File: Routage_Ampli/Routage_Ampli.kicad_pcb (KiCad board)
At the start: 2 copper layers, 110.5 x 100.3 mm, 52 parts, among them J1 Conn_01x03, J2 Conn_01x02, Q1 2N2907, Q10 TIP32, Q11 BD138, Q12 TIP31, Q13 2N2222, Q2 2N2907, Q3 2N2907, Q4 2N2222, Q5 2N2222, Q6 2N2907, Q7 2N2907, Q8 BD139, Q9 BD139, U1 Jack_Mono, U2 Relay_1CT

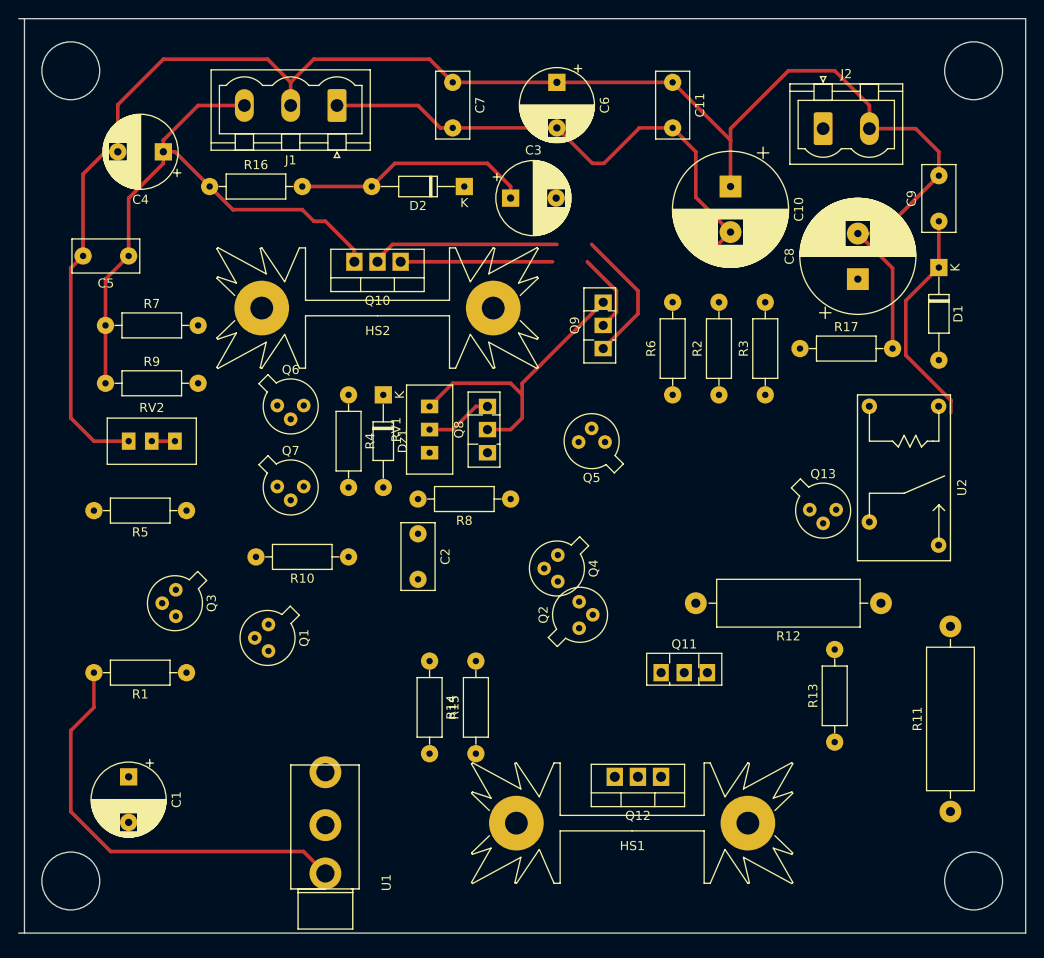
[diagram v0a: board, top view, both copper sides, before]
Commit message: Version avant correction
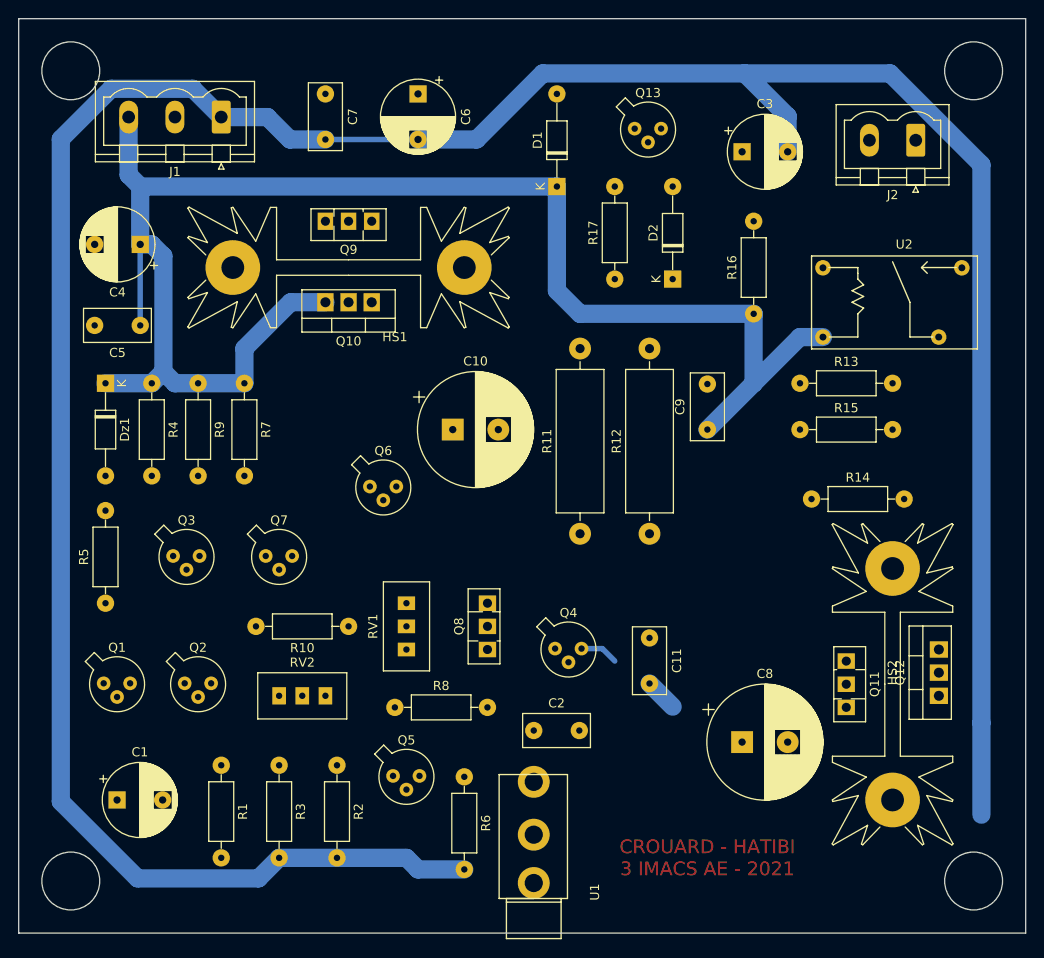
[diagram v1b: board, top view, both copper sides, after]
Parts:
- moved HS2 70.0 mm to (194.3, 115.6), turned to 270 degrees
- moved HS1 68.4 mm to (134.6, 69.8)
- moved R3 67.1 mm to (127.0, 124.5), turned to 270 degrees
- moved R16 61.3 mm to (179.1, 74.9), turned to 90 degrees
- moved C11 61.0 mm to (167.6, 110.5)
- moved R2 58.4 mm to (133.3, 124.5), turned to 270 degrees
- moved C8 52.4 mm to (177.8, 121.9), turned to 0 degrees
- moved R11 50.8 mm to (160.0, 99.1)
- moved R15 50.3 mm to (184.2, 87.6), turned to 0 degrees
- moved R6 47.7 mm to (147.3, 125.7), turned to 270 degrees
- moved Q13 46.0 mm to (166.2, 54.7)
- moved R14 45.5 mm to (185.4, 95.2), turned to 0 degrees
- moved Q2 43.6 mm to (116.8, 115.6), turned to 0 degrees
- moved Q5 43.3 mm to (139.7, 125.7), turned to 0 degrees
- moved D1 42.8 mm to (157.5, 61.0), turned to 90 degrees
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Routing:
- net -12V: track 57.0 -> 320.1 mm
- net GND: track 234.8 -> 0.00 mm
- net +12V: track 91.0 -> 174.5 mm
- net Net-(Q10-Pad2): track 35.7 -> 0.00 mm
- net Net-(Q6-Pad3): track 32.5 -> 0.00 mm
- net Net-(C3-Pad1): track 26.2 -> 0.00 mm
- net Net-(Q10-Pad1): track 25.6 -> 0.00 mm
- net Net-(Q8-Pad3): track 7.40 -> 0.00 mm
- net Net-(C2-Pad1): track 0.00 -> 4.22 mm
- net Net-(R10-Pad2): track 2.54 -> 0.00 mm
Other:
- outline, holes or cut-outs redrawn
- board text added: "CROUARD - HATIBI 3 IMACS AE - 2021"
